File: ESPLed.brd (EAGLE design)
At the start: 70 x 68.8 mm, 27 parts, among them IC1 TLC59711

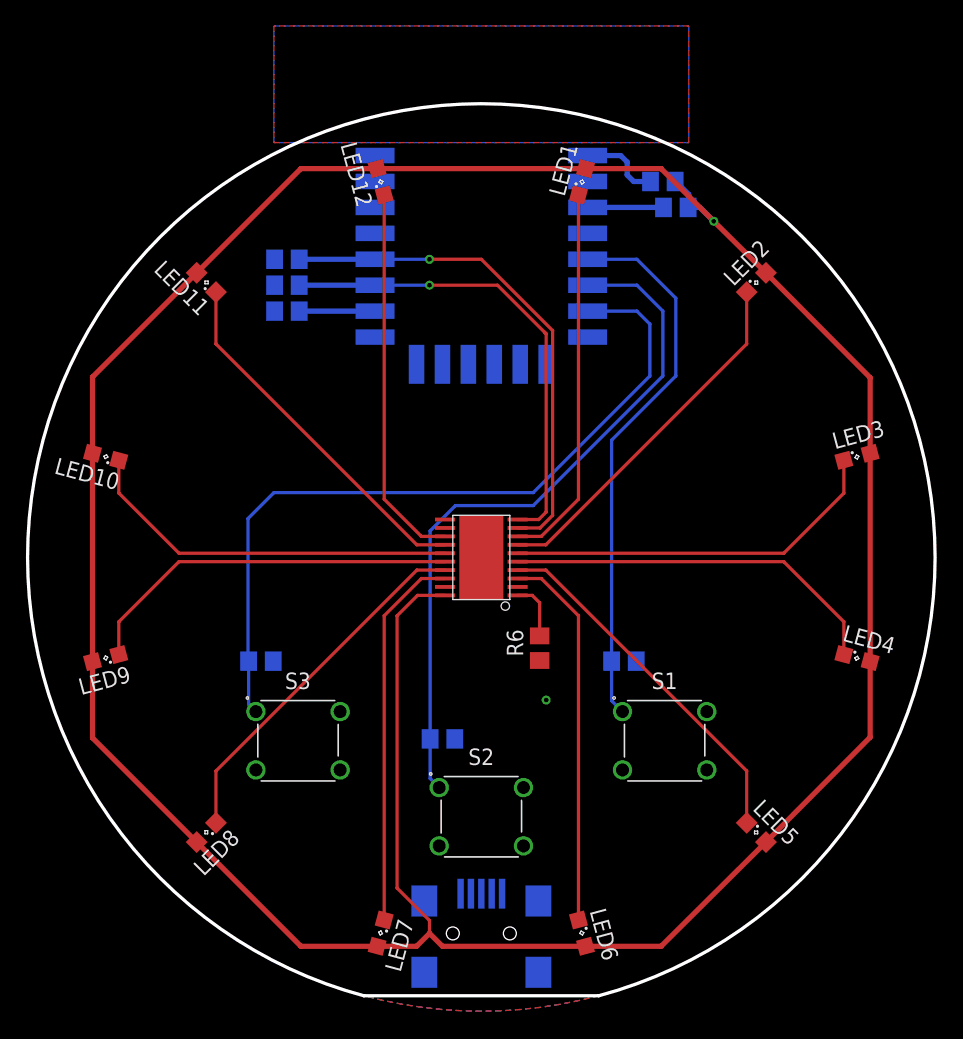
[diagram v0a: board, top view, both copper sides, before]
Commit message: lipo charging
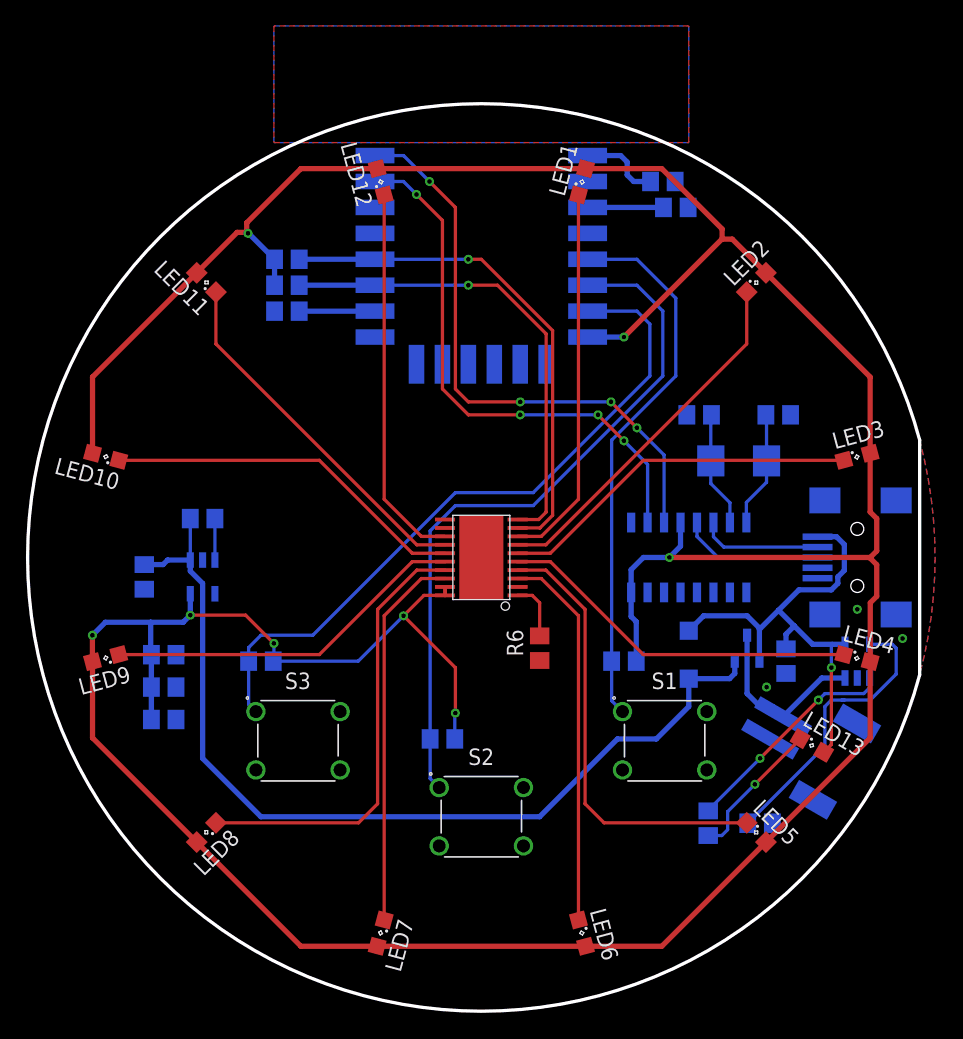
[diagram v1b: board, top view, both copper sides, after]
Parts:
- added C1, C2: 12pF, resistor:C0805
- added C4, C5, C7: 10µF, resistor:C0805
- added C6: 1µF, resistor:C0805
- added D4: MBR120, microbuilder:SOD-123
- added IC2: MCP73831/OT, adafruit:SOT23-5L
- added LED13: (no value), led:SML0805
- added Q1: 12MHz, JonasLib:CX5032GB
- added Q3: DMG3415U, microbuilder:SOT23-R
- added R10: 2k, resistor:R0805
- added R11: 680, resistor:R0805
- added R13, R14: 100k, resistor:R0805
- added U$1: CH340G, ch340g:SOIC16
- added U3: AP2112-3.3, microbuilder:SOT23-5
- added X1: JSTPH, microbuilder:JSTPH2
- moved CN1 42.4 mm to (30.0, 0.00), turned to 270 degrees
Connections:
- net N$1 renamed IREF
- net N$8 renamed GPIO5
- removed net VCC: IC1.19
- new net IN: C4.2, D4.C, Q3.2, R13.1, U3.1
- new net N$1: LED13.C, R11.1
- new net PROG: IC2.5, R10.1
- new net STAT: IC2.1, R11.2
- new net USB_D+: CN1.D+, U$1.5
- new net USB_D-: CN1.D-, U$1.6
- new net USB_RX: U$1.3, U1.TXD0
- new net USB_TX: U$1.2, U1.RXD0
- new net VBAT: IC2.3, Q3.3, X1.2
- new net VREG_EN: R13.2, U3.3
- new net XI: C2.2, Q1.P$1, U$1.7
- new net XO: C1.2, Q1.P$2, U$1.8
- net +3V3: now also C5.2, C6.2, C7.2, IC1.19, U$1.16, U$1.4, U3.5
- net GND: now also C1.1, C2.1, C4.1, C5.1, C6.1, C7.1, IC2.2, R10.2, R14.1, U$1.1, U3.2, X1.1
- net VBUS: now also D4.A, IC2.4, LED13.A, Q3.1, R14.2
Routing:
- net IN: track 0.00 -> 72.3 mm
- net +3V3: track 237.8 -> 291.0 mm, vias 1 -> 8
- net USB_RX: track 0.00 -> 45.3 mm, vias 0 -> 4
- net USB_TX: track 0.00 -> 42.2 mm, vias 0 -> 4
- net VBUS: track 0.00 -> 38.8 mm, vias 0 -> 1
- net PROG: track 0.00 -> 22.2 mm
- net STAT: track 0.00 -> 17.2 mm, vias 0 -> 2
- net VBAT: track 0.00 -> 14.0 mm
- net USB_D+: track 0.00 -> 11.0 mm
- net N$1: track 0.00 -> 11.0 mm, vias 0 -> 1
- net USB_D-: track 0.00 -> 9.46 mm
- net XO: track 0.00 -> 8.97 mm
- net XI: track 0.00 -> 8.94 mm
- net LED8: track 28.1 -> 34.5 mm
- net LED5: track 28.1 -> 34.5 mm
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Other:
- board size 70 x 68.8 mm -> 68.8 x 70 mm
